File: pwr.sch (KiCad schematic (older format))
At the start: 53 parts, among them U1 FT601, U10 MIC94310, U4 ECP5, U6 PAM2306, U7 NCP186, U8 MIC94310, U9 MIC94310, X2 CONN_01X08

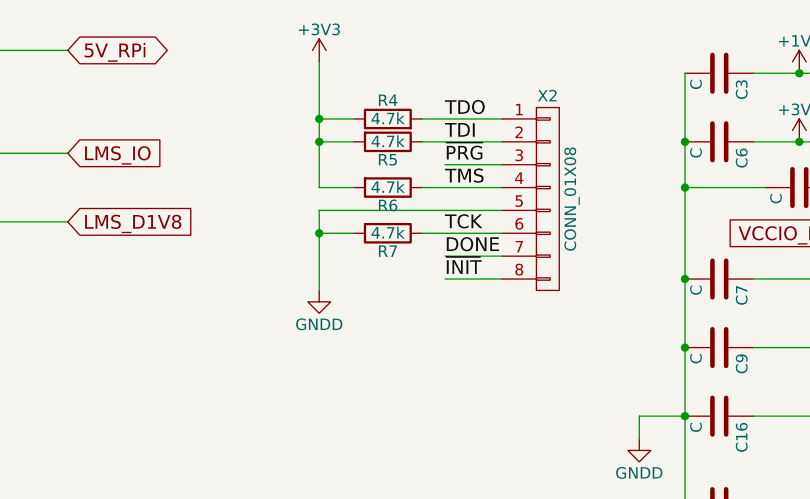
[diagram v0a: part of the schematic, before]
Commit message: Right before Sitch power retracing
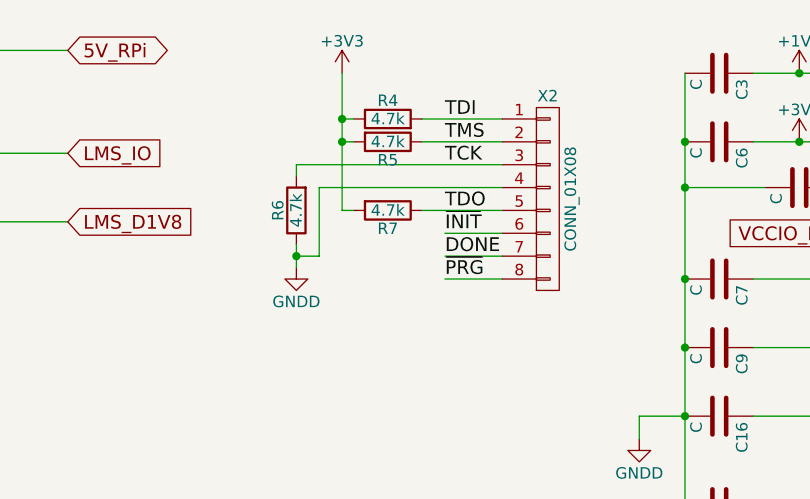
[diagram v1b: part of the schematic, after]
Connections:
- net +3V3: now also R7.2; no longer R6.2
- net GNDD: now also R6.1, X2.4 (P4); no longer R7.2, X2.5 (P5)
- net TCK: now also R6.2, X2.3 (P3); no longer R7.1, X2.6 (P6)
- net TDI: now also R4.2, X2.1 (P1); no longer R5.1, X2.2 (P2)
- net TDO: now also R7.1, X2.5 (P5); no longer R4.2, X2.1 (P1)
- net TMS: now also R5.1, X2.2 (P2); no longer R6.1, X2.4 (P4)
- net ~INIT: now also X2.6 (P6); no longer X2.8 (P8)
- net ~PRG: now also X2.8 (P8); no longer X2.3 (P3)
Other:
- moved on the sheet: R6, R7
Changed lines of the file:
@@
 LIBS:sdr
 LIBS:usb-type-c
+LIBS:sdr-cache
 EELAYER 25 0
 EELAYER END
@@
 L R R7
 U 1 1 589EF8BF
-P 6600 1650
-F 0 "R7" V 6680 1650 50  0000 C CNN
-F 1 "4.7k" V 6600 1650 50  0000 C CNN
-F 2 "Resistors_SMD:R_0603" V 6530 1650 50  0001 C CNN
-F 3 "" H 6600 1650 50  0000 C CNN
-	1    6600 1650
+P 6600 1550
+F 0 "R7" V 6680 1550 50  0000 C CNN
+F 1 "4.7k" V 6600 1550 50  0000 C CNN
+F 2 "Resistors_SMD:R_0603" V 6530 1550 50  0001 C CNN
+F 3 "" H 6600 1550 50  0000 C CNN
+	1    6600 1550
 	0    1    1    0
 $EndComp
@@
 L GNDD #PWR013
 U 1 1 589F005F
-P 6300 1900
-F 0 "#PWR013" H 6300 1650 50  0001 C CNN
-F 1 "GNDD" H 6300 1750 50  0000 C CNN
-F 2 "" H 6300 1900 50  0000 C CNN
-F 3 "" H 6300 1900 50  0000 C CNN
-	1    6300 1900
+P 6200 1800
+F 0 "#PWR013" H 6200 1550 50  0001 C CNN
+F 1 "GNDD" H 6200 1650 50  0000 C CNN
+F 2 "" H 6200 1800 50  0000 C CNN
+F 3 "" H 6200 1800 50  0000 C CNN
+	1    6200 1800
 	1    0    0    -1
 $EndComp
@@
 Text Label 9950 1150 0    60   ~ 0
 TCK
+Text Label 6850 1550 0    60   ~ 0
+TDO
 Text Label 6850 1150 0    60   ~ 0
-TDO
-Text Label 6850 1250 0    60   ~ 0
 TDI
-Text Label 6850 1350 0    60   ~ 0
+Text Label 6850 1850 0    60   ~ 0
 ~PRG
 Text Label 9900 1700 0    60   ~ 0
@@
 Text Label 6850 1750 0    60   ~ 0
 DONE
-Text Label 6850 1850 0    60   ~ 0
+Text Label 6850 1650 0    60   ~ 0
 ~INIT
-Text Label 6850 1650 0    60   ~ 0
+Text Label 6850 1350 0    60   ~ 0
 TCK
-Text Label 6850 1450 0    60   ~ 0
+Text Label 6850 1250 0    60   ~ 0
 TMS
 $Comp
@@
 L R R6
 U 1 1 589F2A11
-P 6600 1450
-F 0 "R6" V 6680 1450 50  0000 C CNN
-F 1 "4.7k" V 6600 1450 50  0000 C CNN
-F 2 "Resistors_SMD:R_0603" V 6530 1450 50  0001 C CNN
-F 3 "" H 6600 1450 50  0000 C CNN
-	1    6600 1450
-	0    1    1    0
+P 6200 1550
+F 0 "R6" V 6280 1550 50  0000 C CNN
+F 1 "4.7k" V 6200 1550 50  0000 C CNN
+F 2 "Resistors_SMD:R_0603" V 6130 1550 50  0001 C CNN
+F 3 "" H 6200 1550 50  0000 C CNN
+	1    6200 1550
+	-1   0    0    1
 $EndComp
 Text Notes 10000 2850 0    60   ~ 0
@@
 	9850 1250 9950 1250
 Wire Wire Line
-	6750 1650 7100 1650
-Wire Wire Line
 	7100 1750 6850 1750
 Wire Wire Line
 	6850 1850 7100 1850
-Wire Wire Line
-	6300 1550 7100 1550
-Wire Wire Line
-	6750 1450 7100 1450
-Wire Wire Line
-	6750 1150 7100 1150
-Wire Wire Line
-	6750 1250 7100 1250
-Wire Wire Line
-	7100 1350 6850 1350
 Wire Wire Line
 	8650 1550 8650 2850
@@
 	1    0    0    -1
 $EndComp
-Connection ~ 6300 1150
-Wire Wire Line
-	6450 1150 6300 1150
-Connection ~ 6300 1250
-Wire Wire Line
-	6450 1250 6300 1250
-Wire Wire Line
-	6300 1450 6450 1450
-Wire Wire Line
-	6300 900  6300 1450
-Wire Wire Line
-	6300 1900 6300 1550
-Wire Wire Line
-	6450 1650 6300 1650
-Connection ~ 6300 1650
-$Comp
-L +3V3 #PWR?
+$Comp
+L +3V3 #PWR036
 U 1 1 58AEBAC7
-P 6300 900
-F 0 "#PWR?" H 6300 750 50  0001 C CNN
-F 1 "+3V3" H 6300 1040 50  0000 C CNN
-F 2 "" H 6300 900 50  0000 C CNN
-F 3 "" H 6300 900 50  0000 C CNN
-	1    6300 900
-	1    0    0    -1
-$EndComp
+P 6400 950
+F 0 "#PWR036" H 6400 800 50  0001 C CNN
+F 1 "+3V3" H 6400 1090 50  0000 C CNN
+F 2 "" H 6400 950 50  0000 C CNN
+F 3 "" H 6400 950 50  0000 C CNN
+	1    6400 950
+	1    0    0    -1
+$EndComp
+Wire Wire Line
+	6750 1150 7100 1150
+Wire Wire Line
+	6750 1250 7100 1250
+Wire Wire Line
+	6750 1550 7100 1550
+Wire Wire Line
+	7100 1650 6850 1650
+Wire Wire Line
+	6400 950  6400 1550
+Wire Wire Line
+	6400 1550 6450 1550
+Wire Wire Line
+	6450 1250 6400 1250
+Connection ~ 6400 1250
+Wire Wire Line
+	6450 1150 6400 1150
+Connection ~ 6400 1150
+Wire Wire Line
+	6200 1350 7100 1350
+Wire Wire Line
+	6200 1400 6200 1350
+Wire Wire Line
+	7100 1450 6300 1450
+Wire Wire Line
+	6300 1450 6300 1750
+Wire Wire Line
+	6200 1700 6200 1800
+Wire Wire Line
+	6300 1750 6200 1750
+Connection ~ 6200 1750
 $EndSCHEMATC
